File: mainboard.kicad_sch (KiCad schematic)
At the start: 34 parts, among them Q2 MMBT3906, Q3 SSM3J332R, Q4 MMBT3906, U3 NJM2391, U4 MSP2807, U6 IM920sl

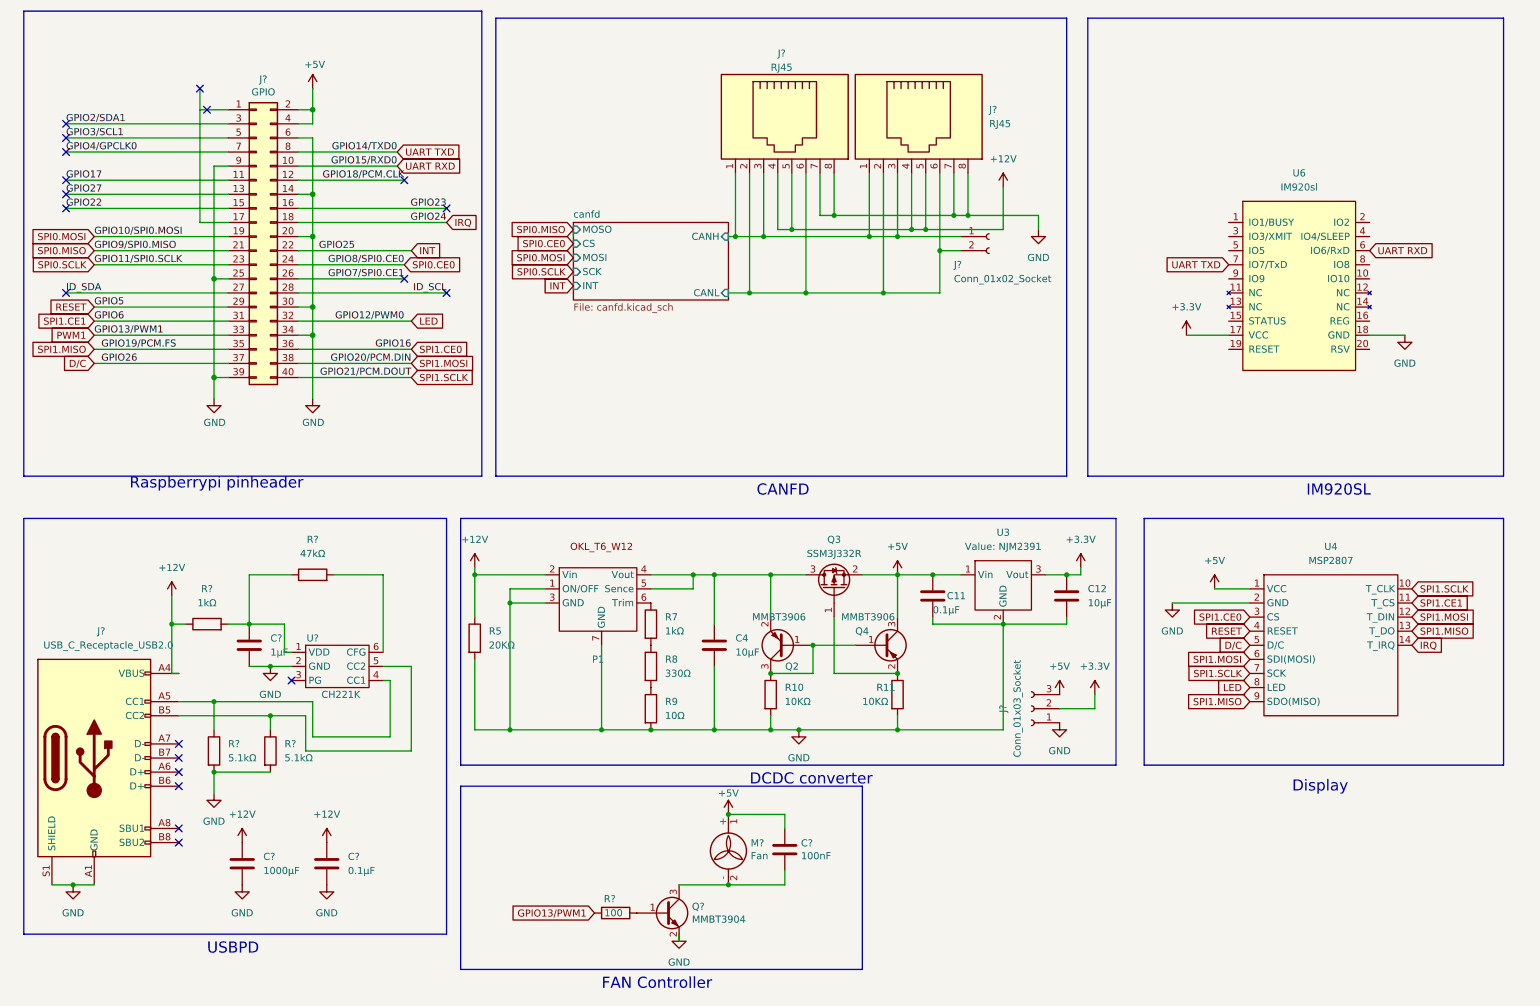
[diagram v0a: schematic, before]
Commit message: first commit
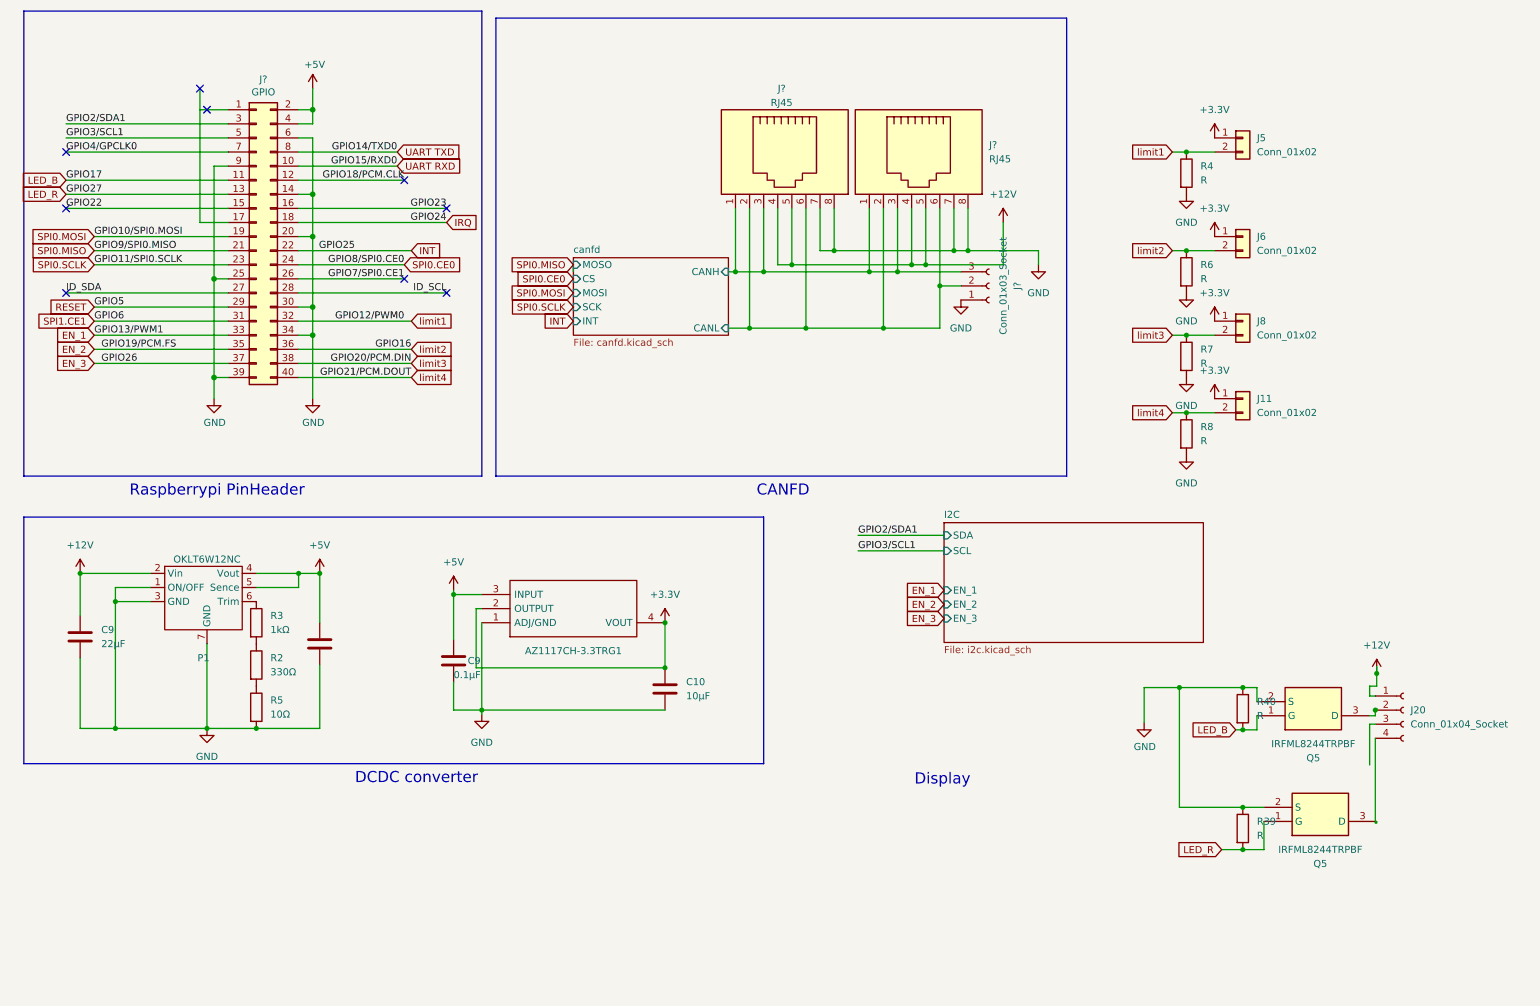
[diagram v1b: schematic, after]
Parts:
- removed C11, C?: 0.1μF, Capacitor_SMD:C_0603_1608Metric_Pad1.08x0.95mm_HandSolder, symbol Device:C
- removed C12: 10µF, Capacitor_SMD:C_0805_2012Metric_Pad1.18x1.45mm_HandSolder, symbol Device:C
- removed C?: 1μF, Capacitor_SMD:C_0805_2012Metric_Pad1.18x1.45mm_HandSolder, symbol Device:C
- removed C?: 1000μF, Capacitor_THT:C_Radial_D10.0mm_H12.5mm_P5.00mm, symbol Device:C
- removed C?: 100nF, Capacitor_SMD:C_0805_2012Metric, symbol Device:C
- removed J?: Conn_01x03_Socket, Connector_PinHeader_2.54mm:PinHeader_1x03_P2.54mm_Vertical, symbol Connector:Conn_01x03_Socket
- removed J?: Conn_01x02_Socket, Connector_PinHeader_2.54mm:PinHeader_1x02_P2.54mm_Vertical, symbol Connector:Conn_01x02_Socket
- removed J?: USB_C_Receptacle_USB2.0, Connector_USB:USB_C_Receptacle_HCTL_HC-TYPE-C-16P-01A, symbol Connector:USB_C_Receptacle_USB2.0
- removed M?: Fan, pihat_cooling:fan_30mm, symbol Motor:Fan
- removed Q2, Q4: MMBT3906, Package_TO_SOT_SMD:SOT-23, symbol Transistor_BJT:MMBT3906
- removed Q3: SSM3J332R, Package_TO_SOT_SMD:SOT-23, symbol Device:Q_PMOS_GSD
- removed Q?: MMBT3904, Package_TO_SOT_SMD:SOT-23, symbol Transistor_BJT:MMBT3904
- removed R10, R11: 10KΩ, Resistor_SMD:R_0805_2012Metric_Pad1.20x1.40mm_HandSolder, symbol Device:R
- removed R5: 20KΩ, Resistor_SMD:R_0805_2012Metric_Pad1.20x1.40mm_HandSolder, symbol Device:R
- removed R? (x2): 5.1kΩ, Resistor_SMD:R_0805_2012Metric_Pad1.20x1.40mm_HandSolder, symbol Device:R
- removed R?: 100, Resistor_SMD:R_0805_2012Metric_Pad1.20x1.40mm_HandSolder, symbol Device:R
- removed R?: 47kΩ, Resistor_SMD:R_0805_2012Metric_Pad1.20x1.40mm_HandSolder, symbol Device:R
- removed R?: 1kΩ, Resistor_SMD:R_0805_2012Metric_Pad1.20x1.40mm_HandSolder, symbol Device:R
- removed U3: NJM2391, Package_TO_SOT_SMD:TO-252-2, symbol regulator:NJM2845DL1
- removed U4: MSP2807, MSP2807:MSP2807, symbol display:MSP2807
- removed U6: IM920sl, interplan:IM920s, symbol interplan:IM920s
- removed U?: CH221K, Package_TO_SOT_SMD:SOT-23-6, symbol CH:CH221K
- added C10: 10µF, Capacitor_SMD:C_0805_2012Metric_Pad1.18x1.45mm_HandSolder, symbol Device:C
- added C9: 0.1μF, Capacitor_SMD:C_0603_1608Metric_Pad1.08x0.95mm_HandSolder, symbol Device:C
- added C9: 22μF, Capacitor_SMD:C_0805_2012Metric_Pad1.18x1.45mm_HandSolder, symbol Device:C
- added IC1: AZ1117CH-3.3TRG1, OKL:SOT230P700X180-4N, symbol SamacSys_Parts:AZ1117CH-3.3TRG1
- added J11, J5, J6, J8: Conn_01x02, Connector_JST:JST_XH_B2B-XH-A_1x02_P2.50mm_Vertical, symbol Connector_Generic:Conn_01x02
- added J20: Conn_01x04_Socket, Connector_JST:JST_XH_B4B-XH-A_1x04_P2.50mm_Vertical, symbol Connector:Conn_01x04_Socket
- added J?: Conn_01x03_Socket, Connector_PinHeader_2.54mm:PinHeader_1x03_P2.54mm_Vertical, symbol Connector:Conn_01x03_Socket
- added Q5 (x2): IRFML8244TRPBF, Package_TO_SOT_SMD:SOT-23-3, symbol SamacSys_Parts:IRFML8244TRPBF
- added R39, R4, R40, R6, R7, R8: R, Resistor_SMD:R_0603_1608Metric_Pad0.98x0.95mm_HandSolder, symbol Device:R
- J? (x2): footprint akiRJ45:7810-8P8C -> OKL:7810-8P8C
- P1: value ~ -> OKLT6W12NC; footprint okL:OKLT6W12NC -> OKL:OKLT6W12NC
- renumbered C4 to C5, R8 to R2, R7 to R3, R9 to R5
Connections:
- net +12V: now also C9.1, J20.1 (Pin_1)
- net +3.3V: now also C10.1, IC1.2 (OUTPUT), IC1.4 (VOUT), J11.1 (Pin_1), J5.1 (Pin_1), J6.1 (Pin_1), J8.1 (Pin_1)
- net +5V: now also C5.1, P1.4 (Vout), P1.5 (Sence), C9.1, IC1.3 (INPUT)
- net GND: now also C10.2, C9.2, C9.2, IC1.1 (ADJ/GND), J?.1 (Pin_1), Q5.2 (S), Q5.2 (S), R39.1, R4.2, R40.1, R6.2, R7.2, R8.2
- net canfd/CANH: now also J?.3 (Pin_3)
- net canfd/CANL: now also J?.2 (Pin_2)
- net D/C renamed EN_3
- net GPIO13/PWM1 renamed EN_1
- net GPIO17 renamed LED_B
- net LED_B: now also Q5.1 (G), R40.2
- net GPIO27 renamed LED_R
- net LED_R: now also Q5.1 (G), R39.2
- net LED renamed limit1
- net limit1: now also J5.2 (Pin_2), R4.1
- net SPI1.CE0 renamed limit2
- net limit2: now also J6.2 (Pin_2), R6.1
- net SPI1.MISO renamed EN_2
- net SPI1.MOSI renamed limit3
- net limit3: now also J8.2 (Pin_2), R7.1
- net SPI1.SCLK renamed limit4
- net limit4: now also J11.2 (Pin_2), R8.1
- new net: J20.2 (Pin_2), Q5.3 (D)
- new net: J20.4 (Pin_4), Q5.3 (D)
- no-connect marks 20 -> 9
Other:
- added sheet I2C (i2c.kicad_sch)
- note added: "Raspberrypi PinHeader"
- note removed: "FAN Controller"
- note removed: "IM920SL"
- note removed: "Raspberrypi pinheader"
- note removed: "USBPD"
- moved on the sheet: J?, R2, R3, R5
